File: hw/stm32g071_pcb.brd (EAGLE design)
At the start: 19 x 38.1 mm, 23 parts, among them IC1 STM32G071

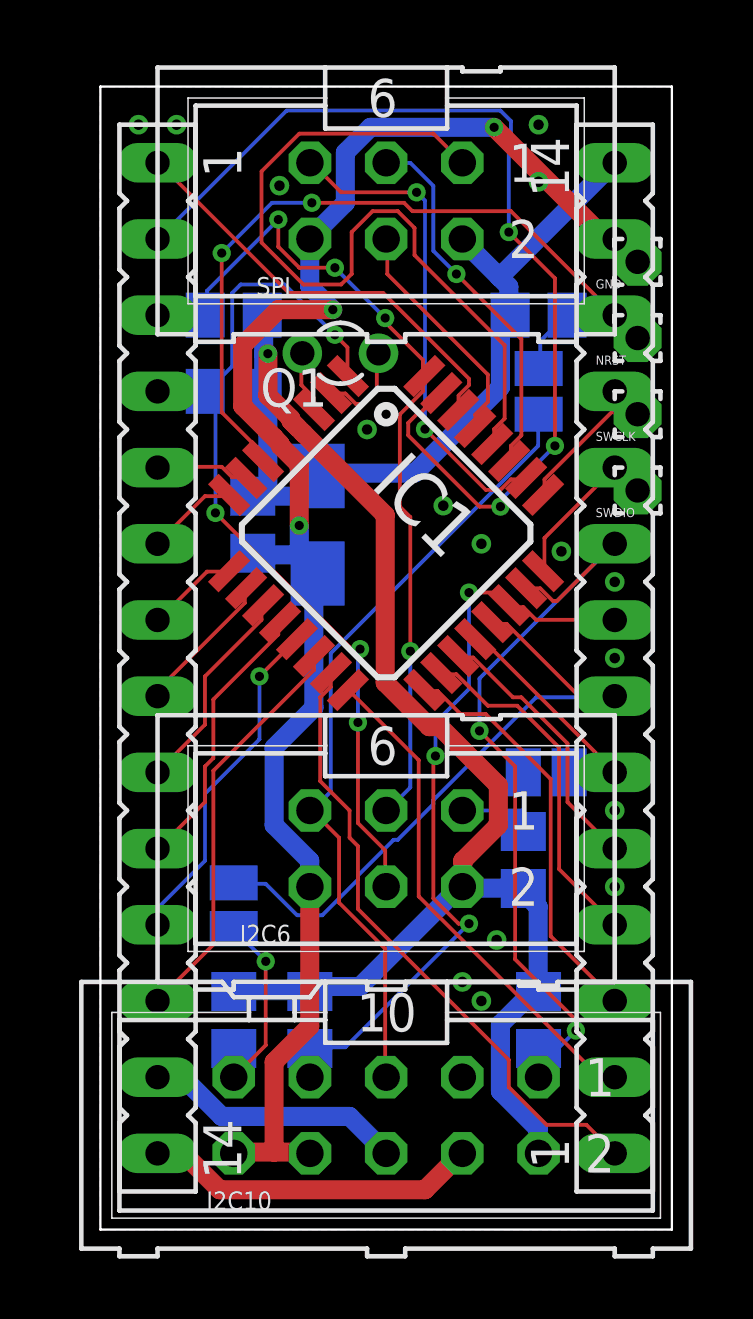
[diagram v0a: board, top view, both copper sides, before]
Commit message: some files updated
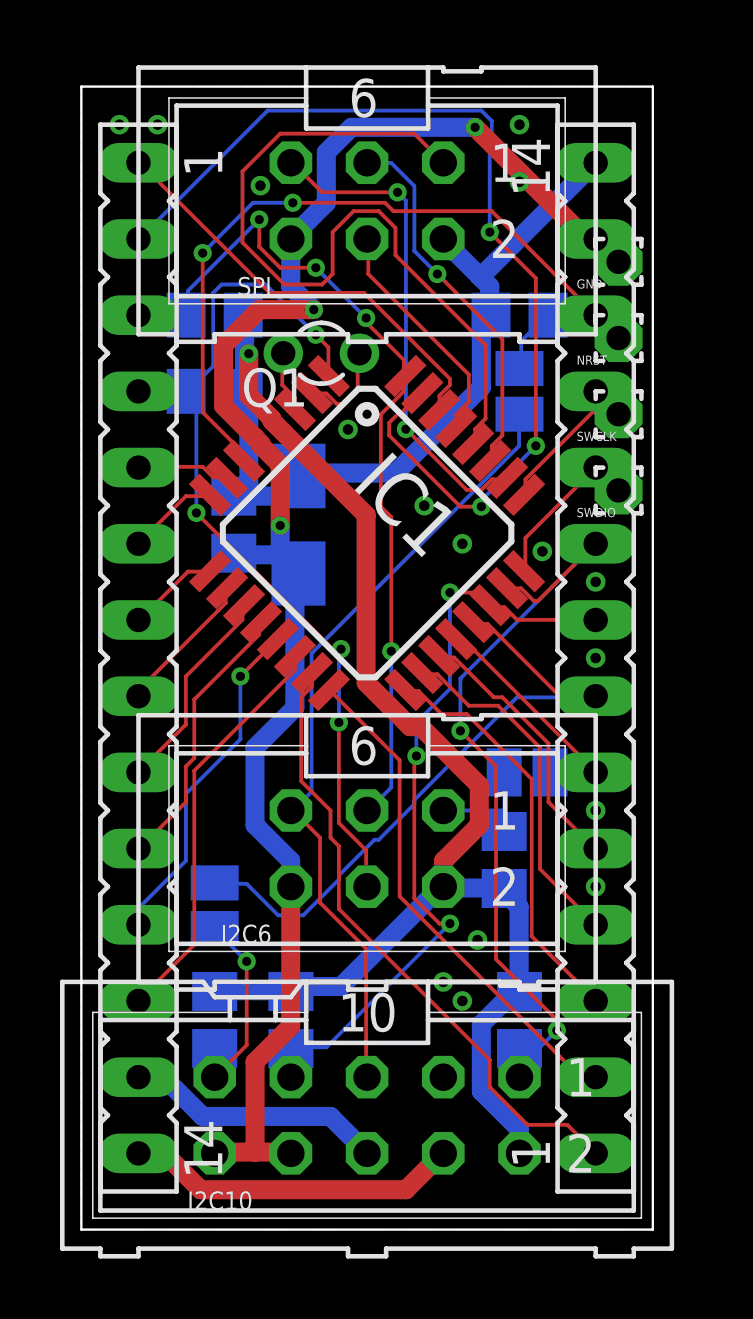
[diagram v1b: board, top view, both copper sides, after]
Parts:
- moved GND 0.64 mm to (17.9, 32.3)
- moved NRST 0.64 mm to (17.9, 29.7)
- moved R 0.64 mm to (17.1, 17.8)
- moved SWCLK 0.64 mm to (17.9, 27.2)
- moved SWDIO 0.64 mm to (17.9, 24.6)
- moved L 0.64 mm to (1.91, 20.3)
- moved C1 0.63 mm to (5.08, 23.5)
- moved C5 0.63 mm to (7.24, 23.5)
- moved I2C10 0.63 mm to (9.53, 3.81)
- moved I2C6 0.63 mm to (9.53, 12.7)
- moved IC1 0.63 mm to (9.53, 27.2)
- moved J_INT1 0.63 mm to (14.9, 15.2)
- moved J_INT2 0.63 mm to (4.45, 10.8)
- moved J_RESET 0.63 mm to (14.6, 27.9)
- moved Q1 0.63 mm to (8.00, 29.2)
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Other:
- board size 19 x 38.1 mm -> 19.1 x 38.1 mm
